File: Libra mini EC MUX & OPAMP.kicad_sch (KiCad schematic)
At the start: 32 parts, among them U6 OPA2365, U7 4052, U8 OPA2365, U9 4052

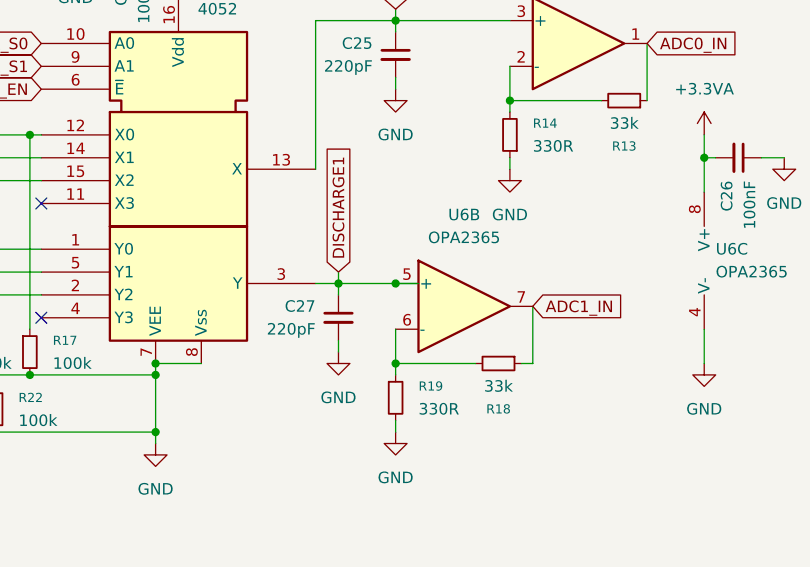
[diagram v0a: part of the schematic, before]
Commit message: 15.04.2026
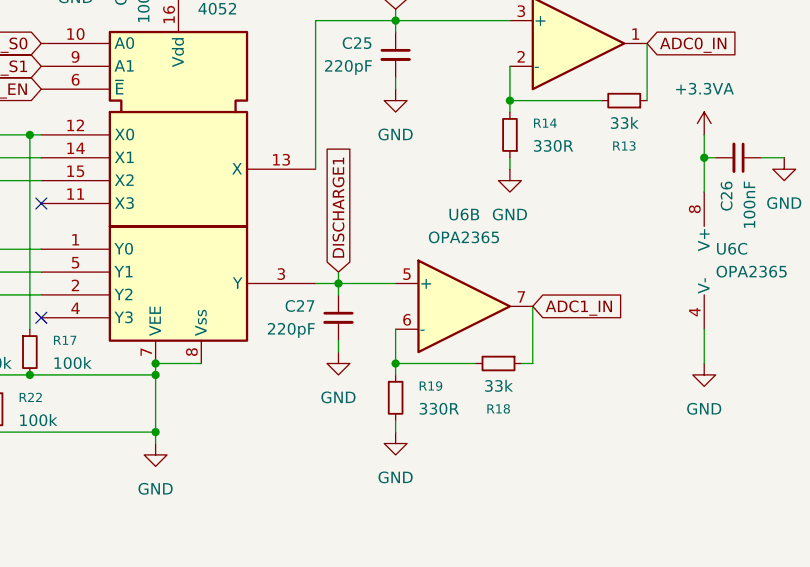
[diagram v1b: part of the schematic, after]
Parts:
- R15, R16, R17, R20, R21, R22, R25, R26, R27, R30, R31, R32: footprint Capacitor_SMD:C_0805_2012Metric -> Resistor_SMD:R_0805_2012Metric
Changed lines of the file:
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@@
 	)
 	(junction
-		(at 104.14 73.66)
-		(diameter 0)
-		(color 0 0 0 0)
-	)
-	(junction
 		(at 116.84 53.34)
 		(diameter 0)
@@
 	(wire
 		(pts
-			(xy 106.68 73.66) (xy 104.14 73.66)
-		)
-		(stroke
-			(width 0)
-			(type default)
-		)
-	)
-	(wire
-		(pts
 			(xy 41.91 90.17) (xy 50.8 90.17)
 		)
@@
 			)
 		)
-		(property "Footprint" "Capacitor_SMD:C_0805_2012Metric"
+		(property "Footprint" "Resistor_SMD:R_0805_2012Metric"
 			(at 49.53 172.72 0)
 			(effects
@@
 			)
 		)
-		(property "Footprint" "Capacitor_SMD:C_0805_2012Metric"
+		(property "Footprint" "Resistor_SMD:R_0805_2012Metric"
 			(at 41.91 87.63 0)
 			(effects
@@
 			)
 		)
-		(property "Footprint" "Capacitor_SMD:C_0805_2012Metric"
+		(property "Footprint" "Resistor_SMD:R_0805_2012Metric"
 			(at 50.8 87.63 0)
 			(effects
@@
 			)
 		)
-		(property "Footprint" "Capacitor_SMD:C_0805_2012Metric"
+		(property "Footprint" "Resistor_SMD:R_0805_2012Metric"
 			(at 54.61 81.28 0)
 			(effects
@@
 			)
 		)
-		(property "Footprint" "Capacitor_SMD:C_0805_2012Metric"
+		(property "Footprint" "Resistor_SMD:R_0805_2012Metric"
 			(at 63.5 81.28 0)
 			(effects
@@
 			)
 		)
-		(property "Footprint" "Capacitor_SMD:C_0805_2012Metric"
+		(property "Footprint" "Resistor_SMD:R_0805_2012Metric"
 			(at 45.72 81.28 0)
 			(effects
@@
 			)
 		)
-		(property "Footprint" "Capacitor_SMD:C_0805_2012Metric"
+		(property "Footprint" "Resistor_SMD:R_0805_2012Metric"
 			(at 58.42 172.72 0)
 			(effects
@@
 			)
 		)
-		(property "Footprint" "Capacitor_SMD:C_0805_2012Metric"
+		(property "Footprint" "Resistor_SMD:R_0805_2012Metric"
 			(at 59.69 87.63 0)
 			(effects
@@
 			)
 		)
-		(property "Footprint" "Capacitor_SMD:C_0805_2012Metric"
+		(property "Footprint" "Resistor_SMD:R_0805_2012Metric"
 			(at 62.23 166.37 0)
 			(effects
@@
 			)
 		)
-		(property "Footprint" "Capacitor_SMD:C_0805_2012Metric"
+		(property "Footprint" "Resistor_SMD:R_0805_2012Metric"
 			(at 67.31 172.72 0)
 			(effects
@@
 			)
 		)
-		(property "Footprint" "Capacitor_SMD:C_0805_2012Metric"
+		(property "Footprint" "Resistor_SMD:R_0805_2012Metric"
 			(at 53.34 166.37 0)
 			(effects
@@
 			)
 		)
-		(property "Footprint" "Capacitor_SMD:C_0805_2012Metric"
+		(property "Footprint" "Resistor_SMD:R_0805_2012Metric"
 			(at 71.12 166.37 0)
 			(effects
